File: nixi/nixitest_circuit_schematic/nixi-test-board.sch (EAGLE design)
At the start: 18 parts, among them IC1 7805T, Q1 MRF136, Q2 2N6107, Q3 BC238

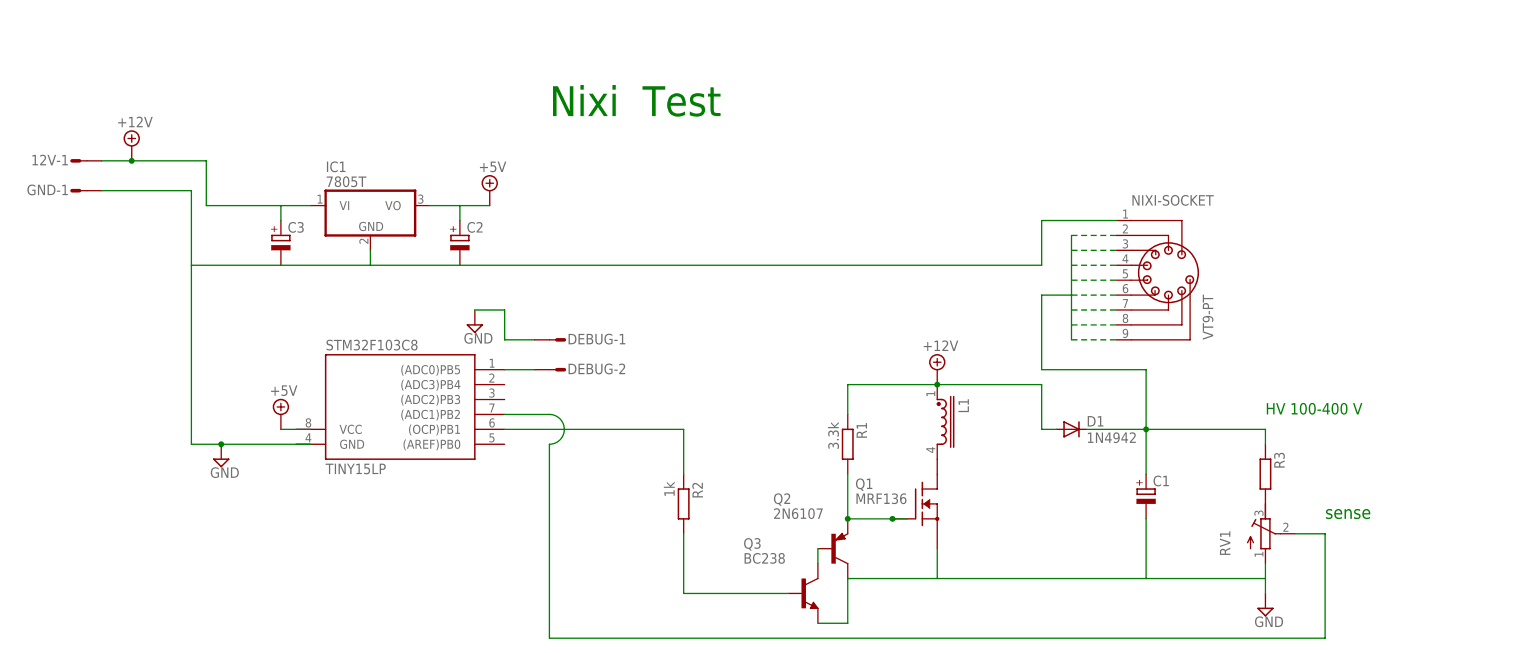
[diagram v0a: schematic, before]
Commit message: reg save
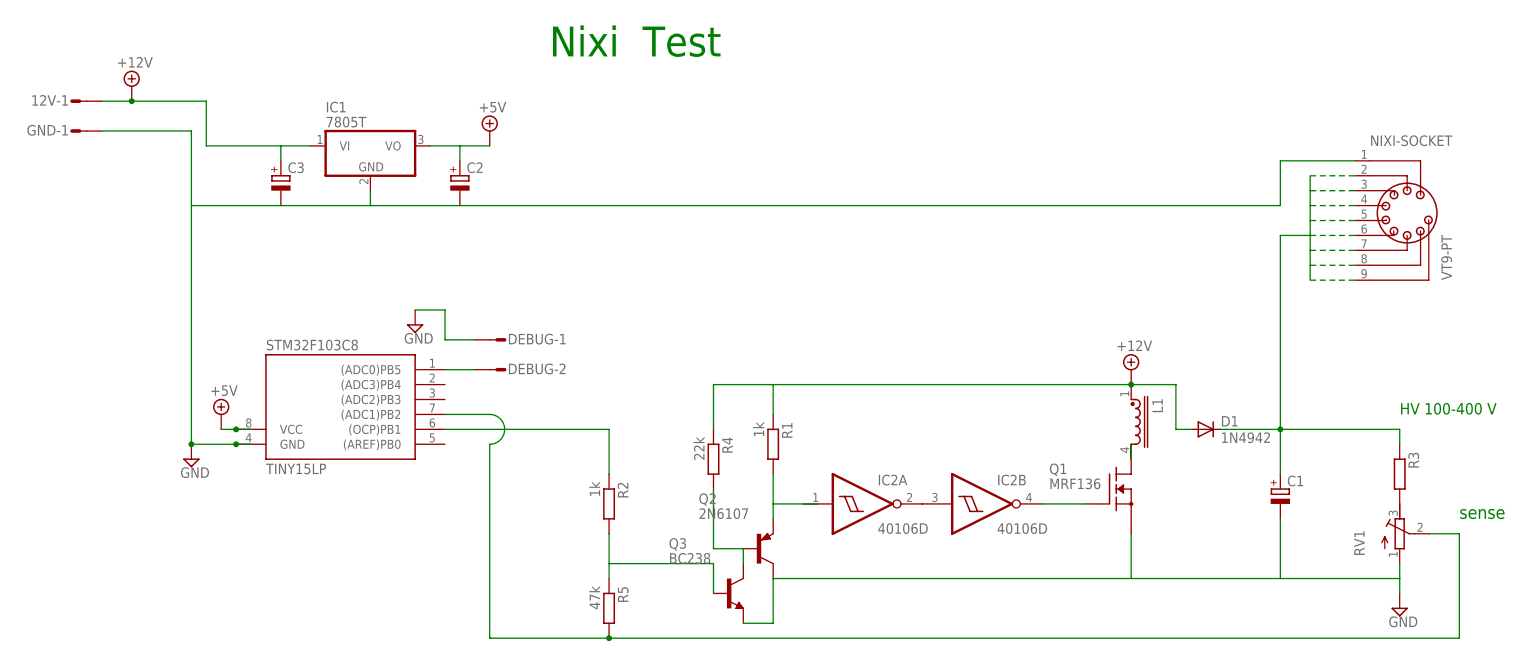
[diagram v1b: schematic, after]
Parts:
- added IC2: 40106D, 40xx:40106D
- added R4: 22k, resistor:R-EU_0207/5V
- added R5: 47k, resistor:R-EU_0207/5V
- R1: value 3.3k -> 1k
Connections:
- new net N$3: IC2B.O, Q1.G
- new net N$9: IC2A.O, IC2B.I
- net +12V: now also R4.1
- net +5V: now also STM32F103C8.VCC
- net GND: now also STM32F103C8.GND
- net N$10: no longer Q1.G
- net N$5: now also R5.2
- net N$6: now also R4.2
- net N$8: now also R5.1
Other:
- moved on the sheet: 12V-1, C1, C2, C3, D1, DEBUG-1, DEBUG-2, GND-1, IC1, L1, NIXI-SOCKET, Q1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

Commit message: reg save
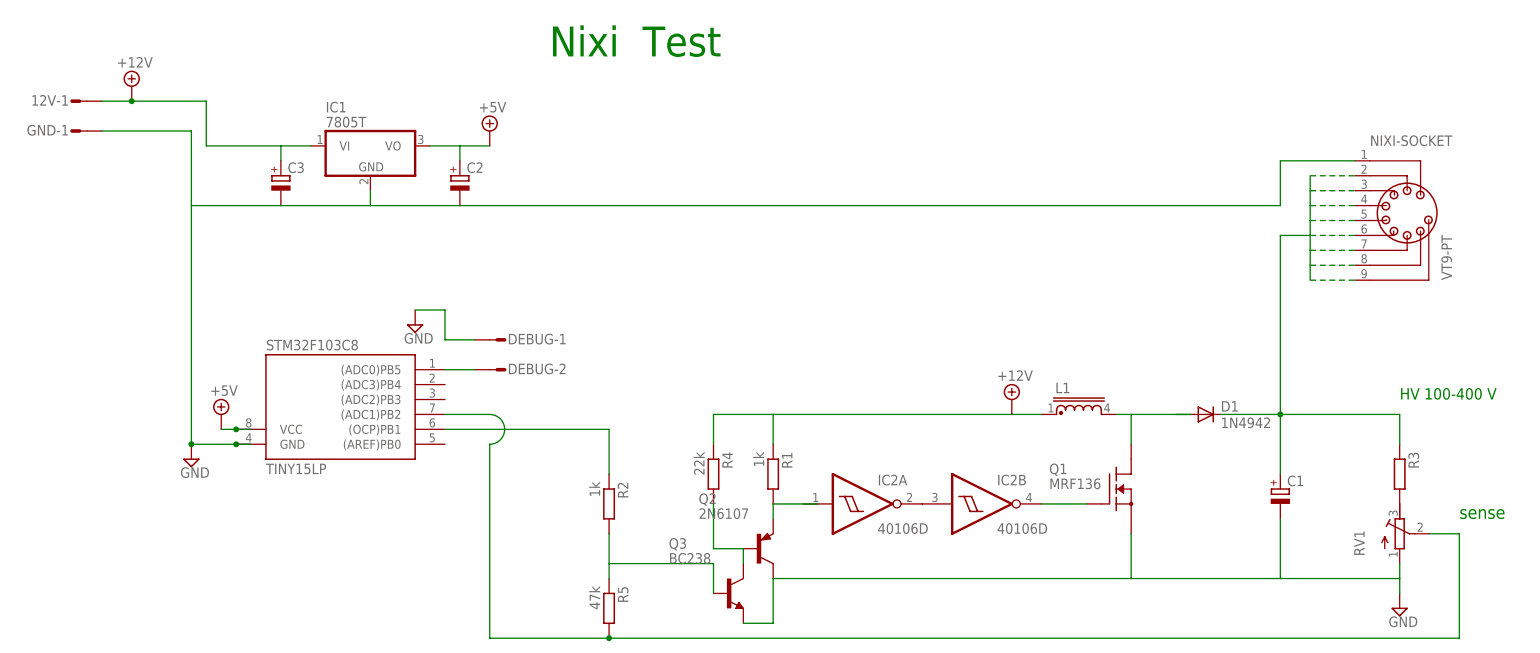
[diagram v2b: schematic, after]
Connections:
- net +12V: no longer D1.A
- net N$2: now also D1.A
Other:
- moved on the sheet: D1, L1, R1, R4
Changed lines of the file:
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@@
 <plain>
 <text x="203.2" y="27.94" size="2.1844" layer="91">sense</text>
-<text x="193.04" y="45.72" size="1.9304" layer="91">HV 100-400 V</text>
+<text x="193.04" y="48.26" size="1.9304" layer="91">HV 100-400 V</text>
 <text x="48.26" y="106.68" size="5.08" layer="91">Nixi  Test</text>
 <frame x1="-50.8" y1="-2.54" x2="213.36" y2="119.38" columns="8" rows="5" layer="116" border-left="no" border-top="no" border-right="no" border-bottom="no"/>
@@
 <instance part="SUPPLY3" gate="+5V" x="38.1" y="93.98"/>
 <instance part="SUPPLY4" gate="+5V" x="-7.62" y="45.72"/>
-<instance part="L1" gate="G$1" x="147.32" y="45.72" rot="R270"/>
-<instance part="D1" gate="1" x="160.02" y="43.18"/>
+<instance part="L1" gate="G$1" x="137.16" y="45.72"/>
+<instance part="D1" gate="1" x="160.02" y="45.72"/>
 <instance part="C1" gate="G$1" x="172.72" y="33.02"/>
 <instance part="C2" gate="G$1" x="33.02" y="86.36"/>
@@
 <instance part="DEBUG" gate="-2" x="40.64" y="53.34" rot="MR0"/>
 <instance part="SUPPLY6" gate="GND" x="25.4" y="60.96"/>
-<instance part="SUPPLY5" gate="+12V" x="147.32" y="53.34"/>
+<instance part="SUPPLY5" gate="+12V" x="127" y="48.26"/>
 <instance part="SUPPLY7" gate="GND" x="193.04" y="12.7"/>
 <instance part="GND" gate="-1" x="-33.02" y="93.98"/>
 <instance part="RV1" gate="G$1" x="193.04" y="25.4"/>
 <instance part="Q2" gate="G$1" x="83.82" y="22.86"/>
-<instance part="R1" gate="G$1" x="86.36" y="40.64" rot="R270"/>
+<instance part="R1" gate="G$1" x="86.36" y="35.56" rot="R270"/>
 <instance part="R2" gate="G$1" x="58.42" y="30.48" rot="R270"/>
 <instance part="Q3" gate="G$1" x="78.74" y="15.24"/>
-<instance part="R4" gate="G$1" x="76.2" y="38.1" rot="R270"/>
+<instance part="R4" gate="G$1" x="76.2" y="35.56" rot="R270"/>
 <instance part="R5" gate="G$1" x="58.42" y="12.7" rot="R270"/>
 <instance part="IC2" gate="A" x="101.6" y="30.48"/>
@@
 </segment>
 <segment>
+<pinref part="SUPPLY5" gate="+12V" pin="+12V"/>
 <pinref part="L1" gate="G$1" pin="1"/>
-<pinref part="SUPPLY5" gate="+12V" pin="+12V"/>
-<wire x1="147.32" y1="50.8" x2="154.94" y2="50.8" width="0.1524" layer="91"/>
-<wire x1="154.94" y1="50.8" x2="154.94" y2="43.18" width="0.1524" layer="91"/>
-<pinref part="D1" gate="1" pin="A"/>
-<wire x1="154.94" y1="43.18" x2="157.48" y2="43.18" width="0.1524" layer="91"/>
-<wire x1="147.32" y1="50.8" x2="86.36" y2="50.8" width="0.1524" layer="91"/>
 <pinref part="R1" gate="G$1" pin="1"/>
-<wire x1="86.36" y1="50.8" x2="86.36" y2="45.72" width="0.1524" layer="91"/>
-<junction x="147.32" y="50.8"/>
+<wire x1="86.36" y1="45.72" x2="86.36" y2="40.64" width="0.1524" layer="91"/>
 <pinref part="R4" gate="G$1" pin="1"/>
-<wire x1="76.2" y1="43.18" x2="76.2" y2="50.8" width="0.1524" layer="91"/>
-<wire x1="76.2" y1="50.8" x2="86.36" y2="50.8" width="0.1524" layer="91"/>
+<wire x1="76.2" y1="40.64" x2="76.2" y2="45.72" width="0.1524" layer="91"/>
+<wire x1="76.2" y1="45.72" x2="86.36" y2="45.72" width="0.1524" layer="91"/>
+<wire x1="86.36" y1="45.72" x2="127" y2="45.72" width="0.1524" layer="91"/>
+<wire x1="132.08" y1="45.72" x2="127" y2="45.72" width="0.1524" layer="91"/>
 </segment>
 </net>
@@
 <pinref part="STM32F103C8" gate="G$1" pin="(ADC0)PB5"/>
 <wire x1="35.56" y1="53.34" x2="30.48" y2="53.34" width="0.1524" layer="91"/>
-</segment>
-</net>
-<net name="N$2" class="0">
-<segment>
-<pinref part="Q1" gate="G$1" pin="D"/>
-<pinref part="L1" gate="G$1" pin="4"/>
-<wire x1="147.32" y1="40.64" x2="147.32" y2="38.1" width="0.1524" layer="91"/>
 </segment>
 </net>
@@
 <wire x1="81.28" y1="22.86" x2="81.28" y2="20.32" width="0.1524" layer="91"/>
 <pinref part="R4" gate="G$1" pin="2"/>
-<wire x1="76.2" y1="33.02" x2="76.2" y2="22.86" width="0.1524" layer="91"/>
+<wire x1="76.2" y1="30.48" x2="76.2" y2="22.86" width="0.1524" layer="91"/>
 <wire x1="76.2" y1="22.86" x2="81.28" y2="22.86" width="0.1524" layer="91"/>
 </segment>
@@
 <pinref part="C1" gate="G$1" pin="+"/>
 <pinref part="R3" gate="G$1" pin="1"/>
-<wire x1="193.04" y1="43.18" x2="193.04" y2="40.64" width="0.1524" layer="91"/>
-<wire x1="172.72" y1="43.18" x2="193.04" y2="43.18" width="0.1524" layer="91"/>
-<wire x1="172.72" y1="43.18" x2="172.72" y2="35.56" width="0.1524" layer="91"/>
-<junction x="172.72" y="43.18"/>
-<wire x1="162.56" y1="43.18" x2="172.72" y2="43.18" width="0.1524" layer="91"/>
+<wire x1="193.04" y1="45.72" x2="193.04" y2="40.64" width="0.1524" layer="91"/>
+<wire x1="172.72" y1="45.72" x2="193.04" y2="45.72" width="0.1524" layer="91"/>
+<wire x1="172.72" y1="45.72" x2="172.72" y2="35.56" width="0.1524" layer="91"/>
+<junction x="172.72" y="45.72"/>
+<wire x1="162.56" y1="45.72" x2="172.72" y2="45.72" width="0.1524" layer="91"/>
 <pinref part="D1" gate="1" pin="C"/>
-<wire x1="172.72" y1="43.18" x2="172.72" y2="76.2" width="0.1524" layer="91"/>
+<wire x1="172.72" y1="45.72" x2="172.72" y2="76.2" width="0.1524" layer="91"/>
 <wire x1="177.8" y1="86.36" x2="177.8" y2="83.82" width="0.1524" layer="91"/>
 <wire x1="177.8" y1="83.82" x2="177.8" y2="81.28" width="0.1524" layer="91"/>
@@
 <pinref part="R1" gate="G$1" pin="2"/>
 <pinref part="Q2" gate="G$1" pin="E"/>
-<wire x1="86.36" y1="35.56" x2="86.36" y2="30.48" width="0.1524" layer="91"/>
 <wire x1="86.36" y1="30.48" x2="86.36" y2="27.94" width="0.1524" layer="91"/>
 <wire x1="93.98" y1="30.48" x2="86.36" y2="30.48" width="0.1524" layer="91"/>
 </segment>
 </net>
+<net name="N$2" class="0">
+<segment>
+<pinref part="D1" gate="1" pin="A"/>
+<wire x1="154.94" y1="45.72" x2="157.48" y2="45.72" width="0.1524" layer="91"/>
+<pinref part="L1" gate="G$1" pin="4"/>
+<wire x1="144.78" y1="45.72" x2="147.32" y2="45.72" width="0.1524" layer="91"/>
+<pinref part="Q1" gate="G$1" pin="D"/>
+<wire x1="147.32" y1="45.72" x2="157.48" y2="45.72" width="0.1524" layer="91"/>
+<wire x1="147.32" y1="45.72" x2="147.32" y2="40.64" width="0.1524" layer="91"/>
+</segment>
+</net>
